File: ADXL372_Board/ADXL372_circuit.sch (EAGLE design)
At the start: 38 parts, among them IC1 STM32L051C6, IC4 SI7006-A20-IM, IC5 LP5907MFX-2.5/NOPB, Q2 BSS138W, SW1 DHT-4235A, U1 MX25R1635FM1IL0, U2 ADXL345BCCZ, U3 ADXL372BCCZ-RL7, Y1 16MHZ_X053201602002, Y2 3.2768KHZ

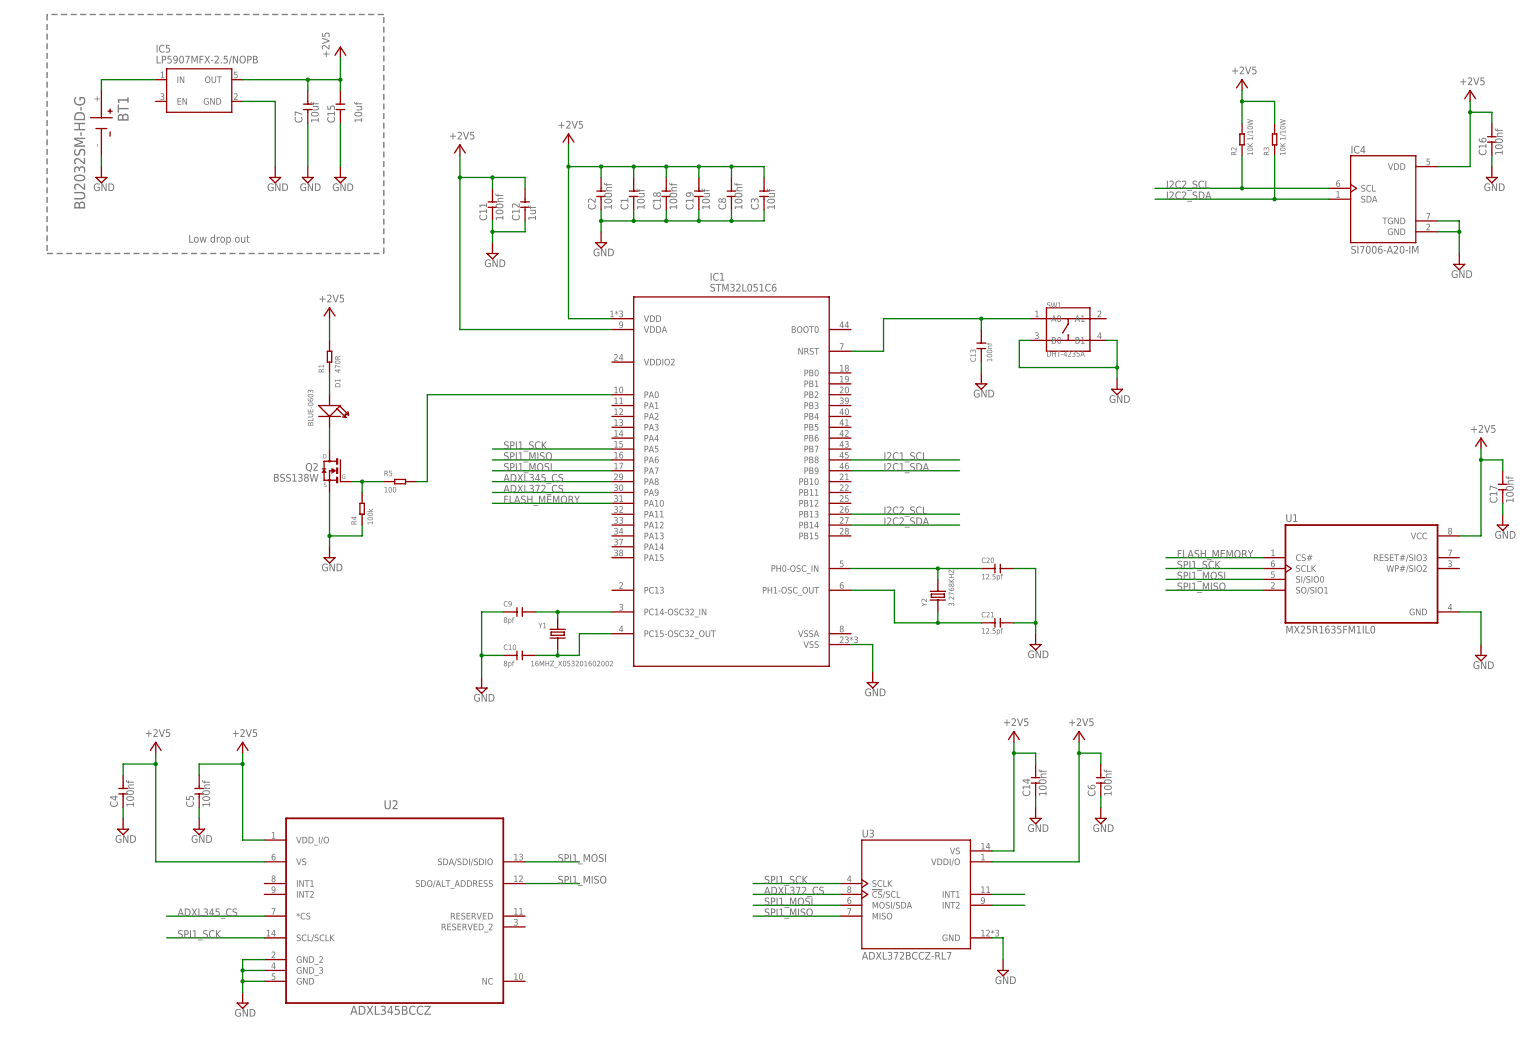
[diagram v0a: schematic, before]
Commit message: Update circuit
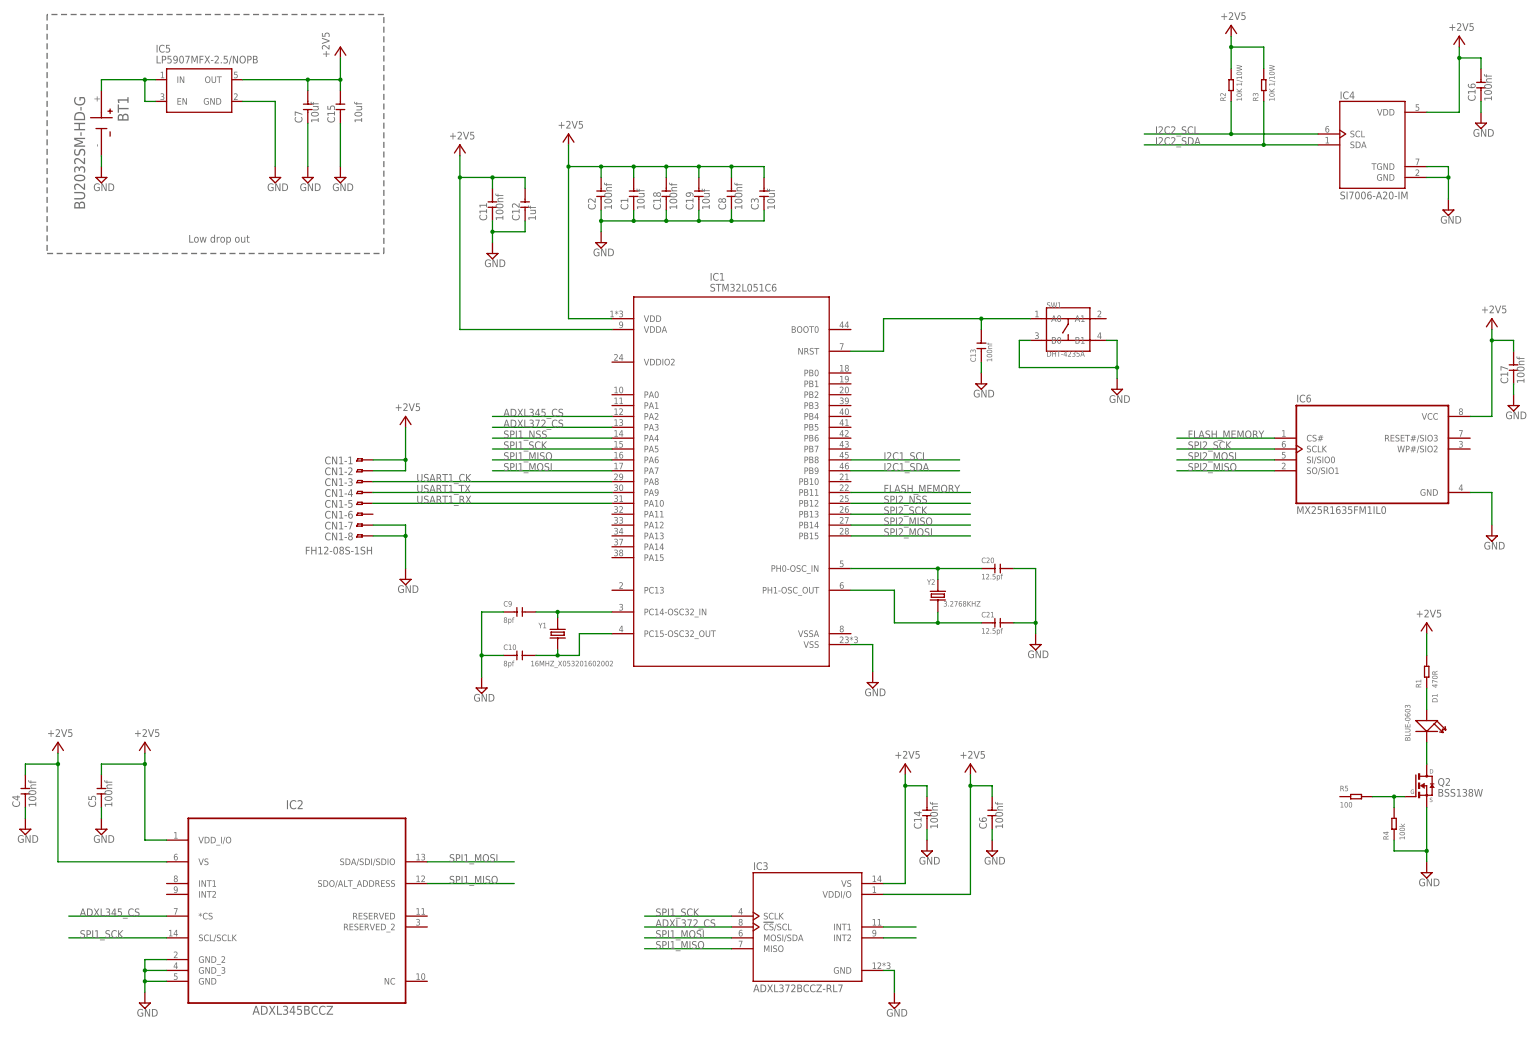
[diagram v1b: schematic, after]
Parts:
- removed U1: MX25R1635FM1IL0, MX25R1635FM1IL0:MX25R1635FM1IL0
- removed U2: ADXL345BCCZ, ADXL345BCCZ:ADXL345BCCZ
- removed U3: ADXL372BCCZ-RL7, ADXL372BCCZ-RL7:ADXL372BCCZ-RL7
- added CN1: FH12-08S-1SH, con-hirose:FH12-08S-1SH
- added IC2: ADXL345BCCZ, ADXL345BCCZ:ADXL345BCCZ
- added IC3: ADXL372BCCZ-RL7, ADXL372BCCZ-RL7:ADXL372BCCZ-RL7
- added IC6: MX25R1635FM1IL0, MX25R1635FM1IL0:MX25R1635FM1IL0
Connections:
- removed net N$10: U2.SDA/SDI/SDIO
- removed net N$11: U2.SDO/ALT_ADDRESS
- removed net N$17: IC1.PA0, R5.2
- removed net N$20: Q2.G, R4.2, R5.1
- removed net N$9: U2.*CS
- new net SPI1_NSS: IC1.PA4
- new net SPI2_MISO: IC1.PB14, IC6.SO/SIO1
- new net SPI2_MOSI: IC1.PB15, IC6.SI/SIO0
- new net SPI2_NSS: IC1.PB12
- new net SPI2_SCK: IC1.PB13, IC6.SCLK
- new net USART1_CK: CN1-3.1, IC1.PA8
- new net USART1_RX: CN1-5.1, IC1.PA10
- new net USART1_TX: CN1-4.1, IC1.PA9
- net +2V5: now also C14.2, C6.2, IC3.VDDI/O, IC3.VS
- net +3V3: now also CN1-1.1, CN1-2.1, IC2.VDD_I/O, IC2.VS, IC6.VCC; no longer C14.2, C6.2, U1.VCC, U2.VDD_I/O, U2.VS, U3.VDDI/O, U3.VS
- net ADXL345_CS: now also IC1.PA2, IC2.*CS; no longer IC1.PA8
- net ADXL372_CS: now also IC1.PA3, IC3.!CS!/SCL; no longer IC1.PA9, U3.!CS!/SCL
- net FLASH_MEMORY: now also IC1.PB11, IC6.CS#; no longer IC1.PA10, U1.CS#
- net GND: now also CN1-7.1, CN1-8.1, IC2.GND, IC2.GND_2, IC2.GND_3, IC3.GND, IC6.GND; no longer U1.GND, U2.GND, U2.GND_2, U2.GND_3, U3.GND
- net I2C2_SCL: no longer IC1.PB13
- net I2C2_SDA: no longer IC1.PB14
- net N$12: now also IC3.INT1; no longer U3.INT1
- net N$13: now also IC3.INT2; no longer U3.INT2
- net N$22: now also IC5.EN
- net N$4: now also Q2.G, R4.2, R5.2; no longer U2.SCL/SCLK
- net SPI1_MISO: now also IC2.SDO/ALT_ADDRESS, IC3.MISO; no longer U1.SO/SIO1, U3.MISO
- net SPI1_MOSI: now also IC2.SDA/SDI/SDIO, IC3.MOSI/SDA; no longer U1.SI/SIO0, U3.MOSI/SDA
- net SPI1_SCK: now also IC2.SCL/SCLK, IC3.SCLK; no longer U1.SCLK, U3.SCLK
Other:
- moved on the sheet: C14, C16, C17, C4, C5, C6, D1, IC4, Q2, R1, R2, R3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

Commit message: update circuit
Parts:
- removed BT1: BU2032SM-HD-G, BU2032SM-HD-G:BU2032SM-HD-G
- removed C15, C7: 10uf, OPL_Capacitor:CERAMIC-10UF-10V-(-20%～+80%)-Y5V(0805)
- removed IC5: LP5907MFX-2.5/NOPB, LP5907MFX-2.5_NOPB:LP5907MFX-2.5/NOPB
- added BT2: BU2032SM-HD-G, BU2032SM-HD-G:BU2032SM-HD-G
- added C22, C24, C25: 10uf, OPL_Capacitor:CERAMIC-10UF-10V-(-20%～+80%)-Y5V(0805)
- added C23: 100nf, OPL_Capacitor:CERAMIC-100NF-50V-10%-X7R(0603)
- added IC7: 74AHC1G14DCK, 74xx-little-us:74AHC1G14DCK
- added IC8: LP5907MFX-2.5/NOPB, LP5907MFX-2.5_NOPB:LP5907MFX-2.5/NOPB
- added R6: 10K 1/10W, OPL_Resistor:SMD-RES-10K-5%-1/10W(0603)
- added SW2: B3U-1000P-2P-SMD, OPL_Switch:SMD-BUTTON(2P-3.0X2.5X1.2+0.4MM)-B3U-1000P-2P-SMD
- added SW3: JS202011SCQN, JS202011SCQN:JS202011SCQN
- added TP1, TP2, TP3, TP4, TP5, TP6, TP7, TP8: TPB1,27, testpad:TPB1,27
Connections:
- removed net N$12: IC3.INT1
- removed net N$13: IC3.INT2
- removed net N$22: BT1.+, IC5.EN, IC5.IN
- new net +BAT: BT2.+, SW3.1, SW3.4
- new net +VIN: IC8.EN, IC8.IN, SW3.2, SW3.5
- new net 345_INT1: IC1.PA1, IC2.INT1
- new net 345_INT2: IC1.PA2, IC2.INT2
- new net 372_INT1: IC1.PB1, IC3.INT1
- new net 372_INT2: IC1.PB2, IC3.INT2
- new net MODE_LED: IC1.PB3, R5.1
- new net MODE_SW: IC1.PB4, IC7A.O
- new net N$10: IC1.PB7, TP7.TP
- new net N$11: IC1.PB10, TP8.TP
- new net N$5: IC7A.I, R6.1, SW2.2
- new net N$6: IC1.PA3, TP3.TP
- new net N$7: IC1.PA15, TP4.TP
- new net N$8: IC1.PB5, TP5.TP
- new net N$9: IC1.PB6, TP6.TP
- new net SYS_SWCLK: IC1.PA14, TP2.TP
- new net SYS_SWDIO: IC1.PA13, TP1.TP
- new net USART1_CTS: CN1-5.1, IC1.PA11
- new net USART1_RTS: CN1-6.1, IC1.PA12
- net +2V5: now also C22.2
- net +3V3: now also C23.2, IC7P.VCC, R6.2, SW3.3, SW3.6; no longer CN1-2.1
- net ADXL345_CS: now also IC1.PA0; no longer IC1.PA2
- net ADXL372_CS: now also IC1.PB0; no longer IC1.PA3
- net GND: now also BT2.-, C22.1, C23.1, C24.1, C25.1, IC7P.GND, IC8.GND, SW2.1; no longer BT1.-, C15.1, C7.1, IC5.GND
- net USART1_CK: now also CN1-2.1; no longer CN1-3.1
- net USART1_RX: now also CN1-4.1; no longer CN1-5.1
- net USART1_TX: now also CN1-3.1; no longer CN1-4.1
- net VCC: now also C24.2, C25.2, IC8.OUT; no longer C15.2, C7.2, IC5.OUT
